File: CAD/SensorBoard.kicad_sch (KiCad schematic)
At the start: 78 parts, among them J1 USB C 2.0, J2 SWD Connector, J3 UART Connector, J4 DAC Connector, SW1 SW_1, SW2 SW_2, SW3 SW_3, SW4 SW_4, SW5 SW_BOOT, SW6 SW_RST, U1 STM32U073CCT6, U2 MIC5365, U3 USBLC6-2SC6, U4 BME680, U5 BMI323, U6 TC1047, X1 32MHz, X2 32kHz768

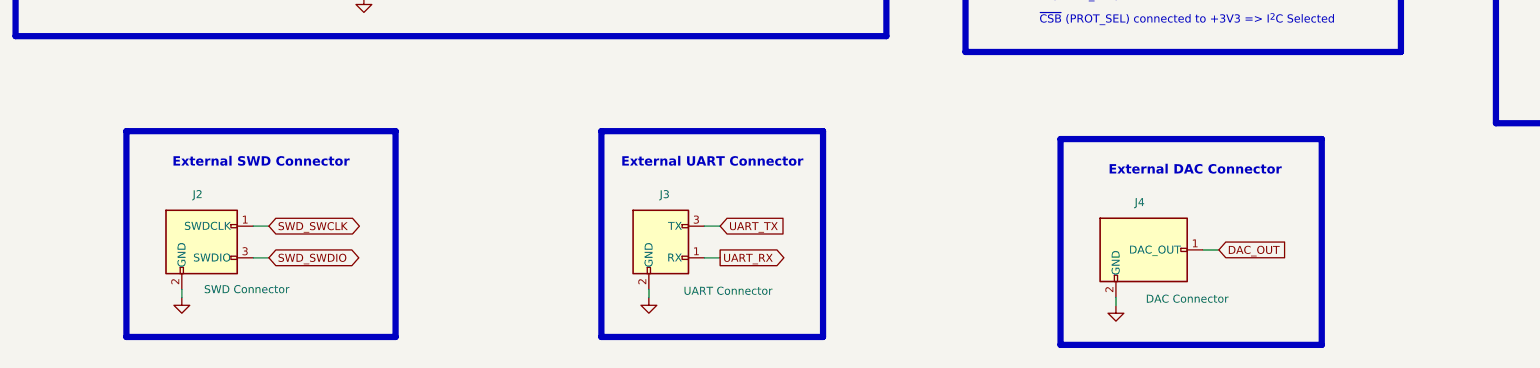
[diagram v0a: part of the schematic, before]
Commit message: Begin initial PCB design
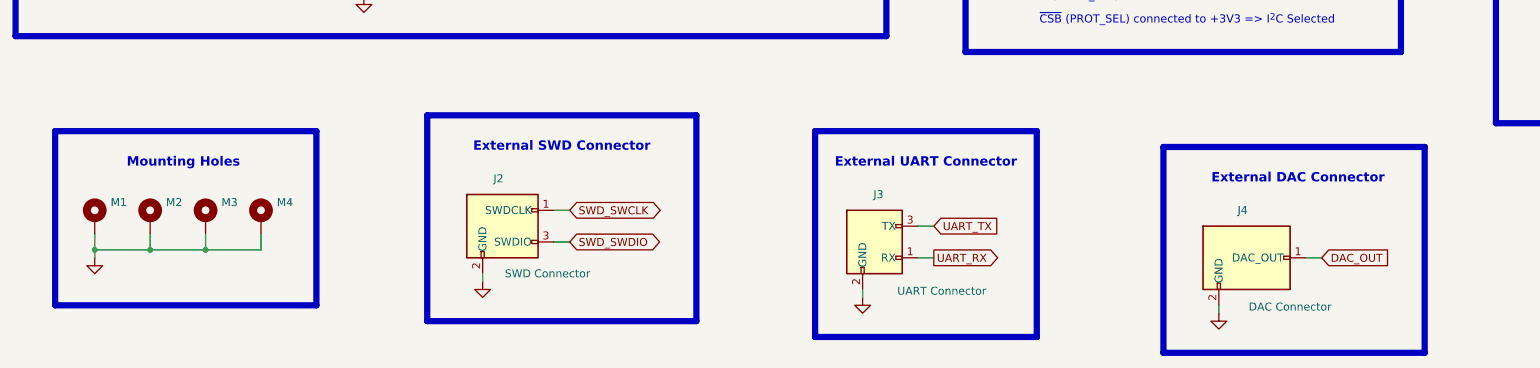
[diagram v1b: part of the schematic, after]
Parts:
- added M1: M1, MountingHole:MountingHole_3.2mm_M3_Pad_Via, symbol Mechanical:MountingHole_Pad
- added M2: M2, MountingHole:MountingHole_3.2mm_M3_Pad_Via, symbol Mechanical:MountingHole_Pad
- added M3: M3, MountingHole:MountingHole_3.2mm_M3_Pad_Via, symbol Mechanical:MountingHole_Pad
- added M4: M4, MountingHole:MountingHole_3.2mm_M3_Pad_Via, symbol Mechanical:MountingHole_Pad
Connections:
- net GND: now also M1.1, M2.1, M3.1, M4.1
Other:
- note added: "Mounting Holes"
- moved on the sheet: J2, J3, J4
